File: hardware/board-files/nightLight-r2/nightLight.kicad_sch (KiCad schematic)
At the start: 41 parts, among them IC1 PAM2401SCADJ, IC2 MCP73123T-22SI_MF, J1 USB_C_Receptacle_PowerOnly_6P, J2 Conn_01x03, J3 Conn_01x03, J4 Conn_01x03, J5 Conn_01x03, J6 Conn_01x05_Pin, SW1 TILT, U2 ATtiny1614-SS

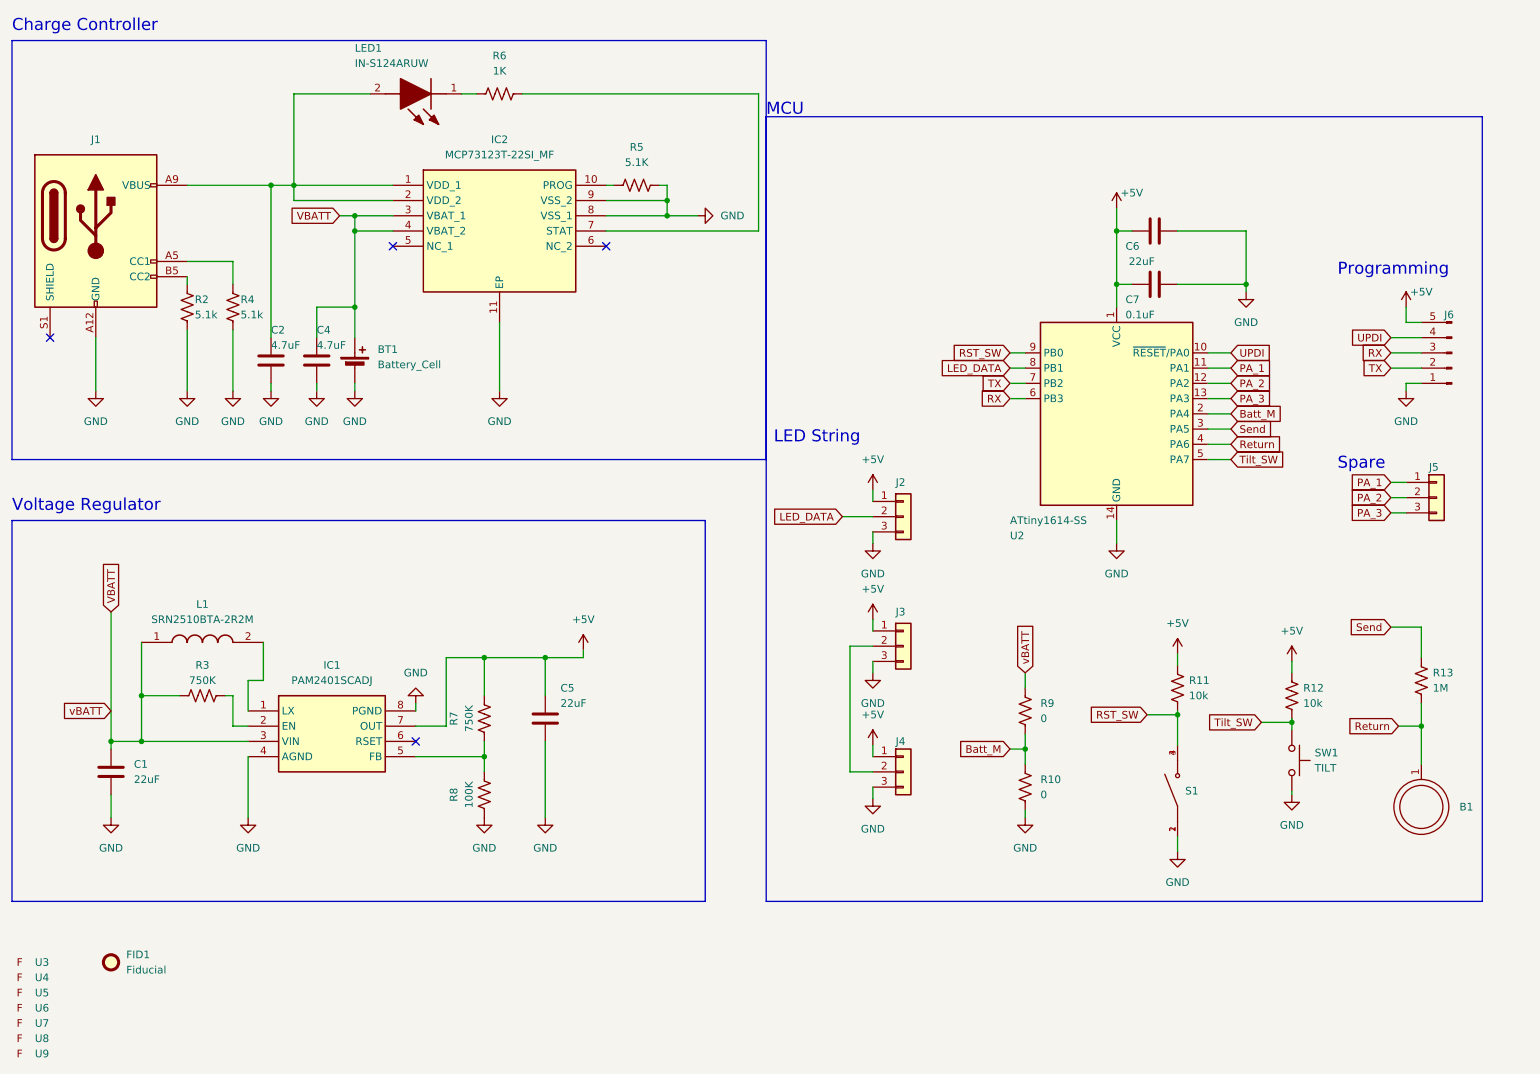
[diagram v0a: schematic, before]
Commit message: messing around during testing
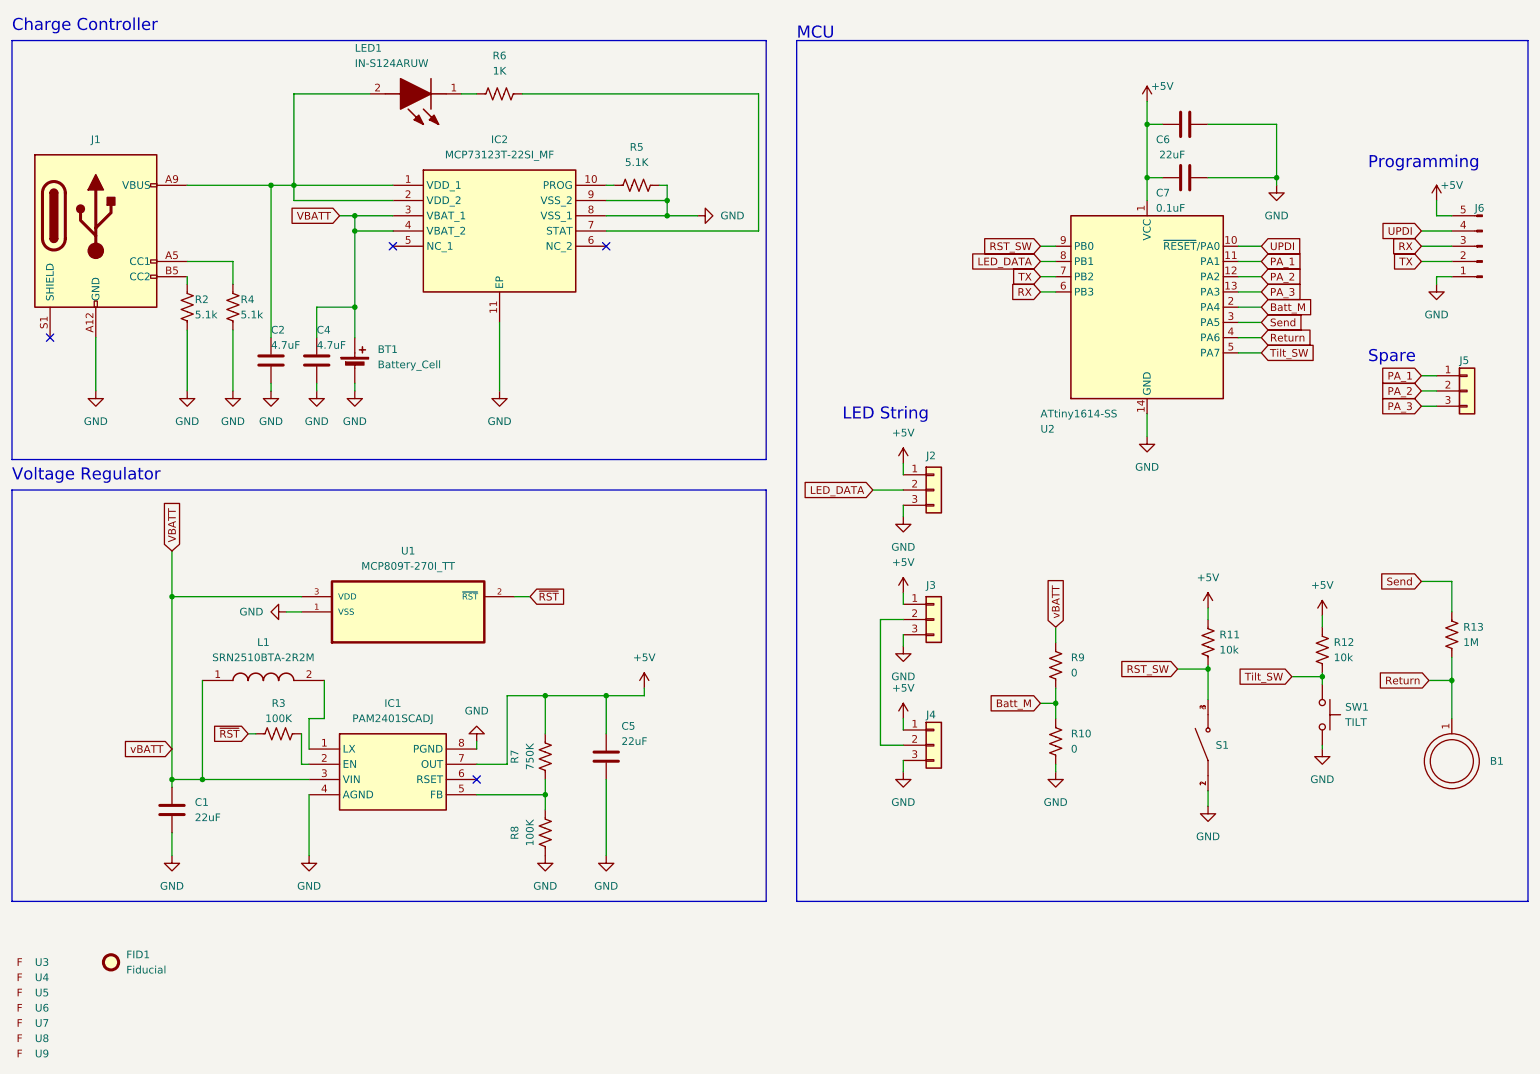
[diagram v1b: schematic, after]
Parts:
- added U1: MCP809T-270I_TT, MCP809T-270I_TT:SOT95P237X112-3N, symbol MCP809T-270I_TT:MCP809T-270I_TT
- R3: value 750K -> 100K
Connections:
- net GND: now also U1.1 (VSS)
- net VBATT: now also U1.3 (VDD); no longer R3.1
- new net ~{RST}: R3.1, U1.2 (~{RST})
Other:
- moved on the sheet: B1, C1, C5, C6, C7, IC1, J2, J3, J4, J5, J6, L1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
